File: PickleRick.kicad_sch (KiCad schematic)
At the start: 83 parts, among them J1 Conn_01x06_Male, J10 Conn_01x03_Male, J11 Conn_01x02_Male, J2 Conn_01x02_Male, J3 Conn_01x02_Male, J4 Micro_SD_Card_Det, J5 292227-7, Q1 MMDT2222A, Q2 PMV20ENR, U1 SN65HVD230, U2 ESP32-WROOM-32D, U3 MS5607-02BA

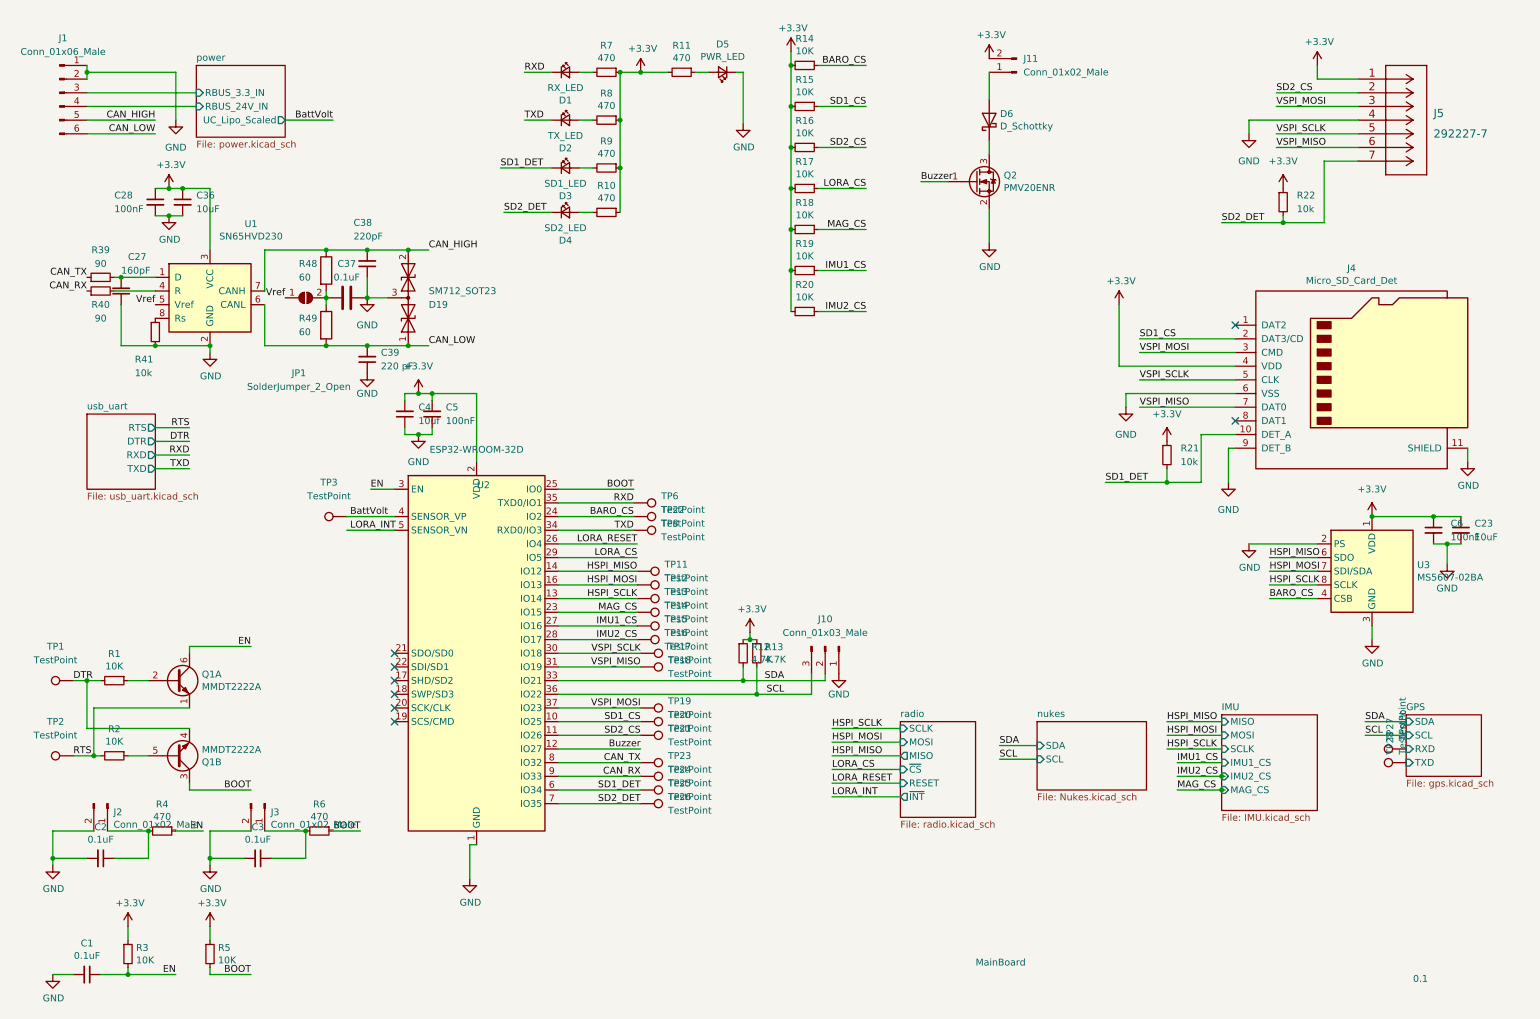
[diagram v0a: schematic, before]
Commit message: working on v2
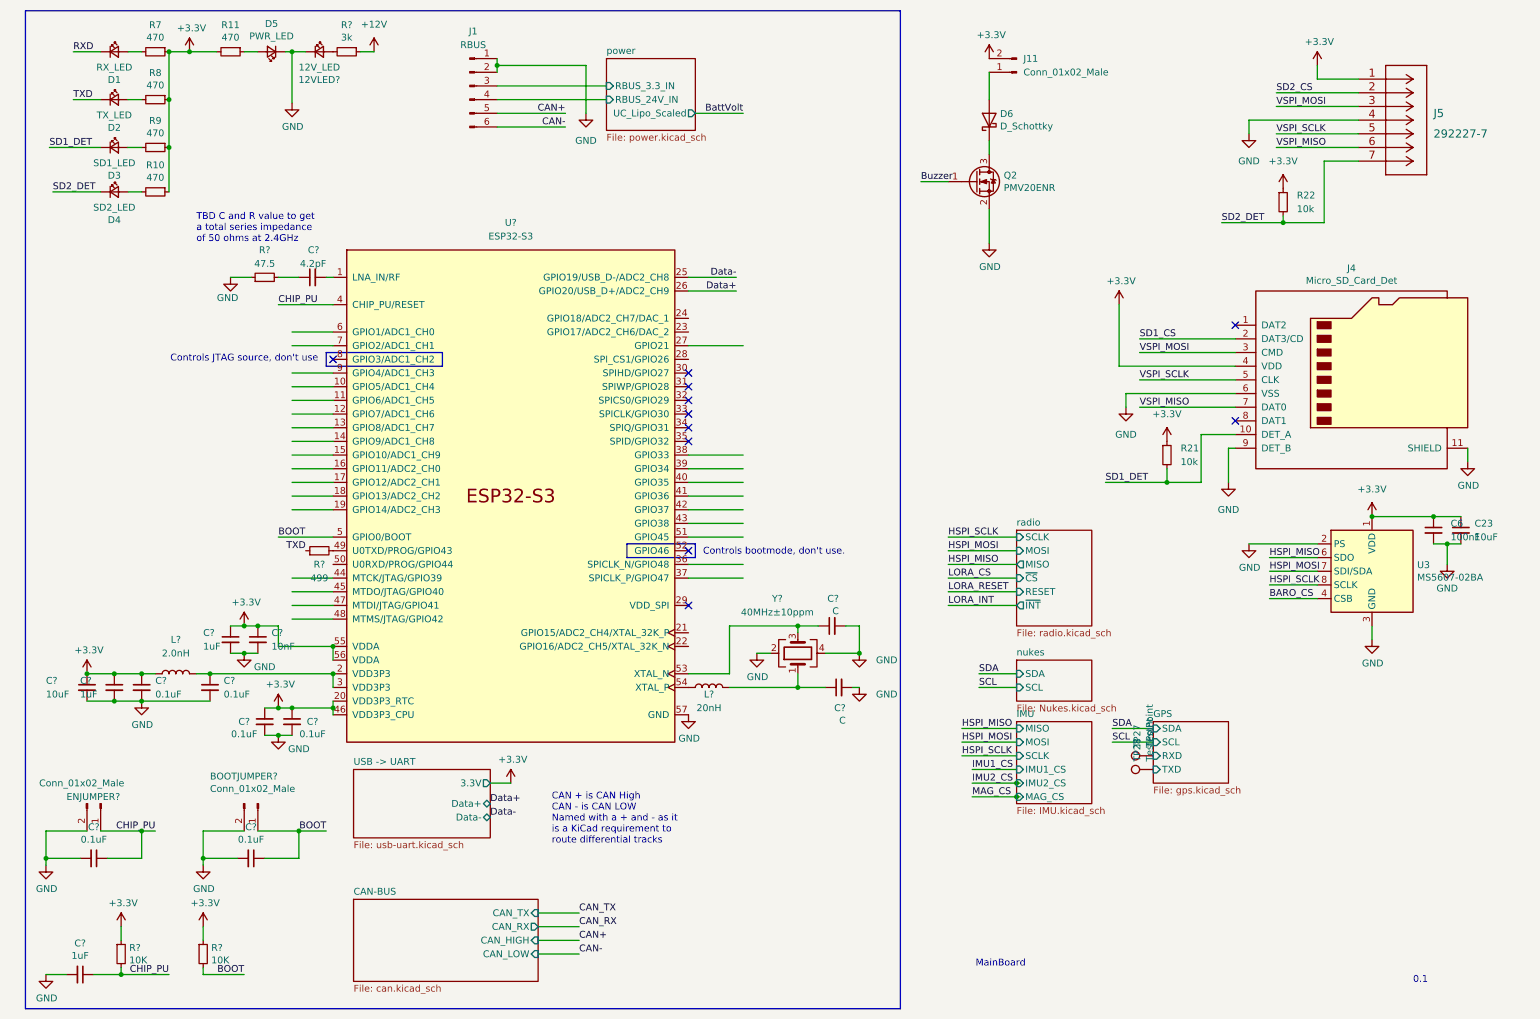
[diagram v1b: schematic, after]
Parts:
- removed C1, C2, C3: 0.1uF, Capacitor_SMD:C_0603_1608Metric, symbol Device:C_Small
- removed C27: 160pF, Capacitor_SMD:C_0603_1608Metric, symbol Device:C_Small
- removed C28, C5: 100nF, Capacitor_SMD:C_0603_1608Metric, symbol Device:C_Small
- removed C36: 10uF, Capacitor_SMD:C_0603_1608Metric, symbol Device:C_Small
- removed C37: 0.1uF, Capacitor_SMD:C_0603_1608Metric, symbol Device:C
- removed C38: 220pF, Capacitor_SMD:C_0603_1608Metric, symbol Device:C_Small
- removed C39: 220 pF, Capacitor_SMD:C_0603_1608Metric, symbol Device:C_Small
- removed C4: 10uf, Capacitor_SMD:C_0603_1608Metric, symbol Device:C_Small
- removed D19: SM712_SOT23, Package_TO_SOT_SMD:SOT-23, symbol Diode:SM712_SOT23
- removed J10: Conn_01x03_Male, Connector_PinHeader_2.54mm:PinHeader_1x03_P2.54mm_Vertical, symbol Connector:Conn_01x03_Male
- removed J2, J3: Conn_01x02_Male, Connector_PinHeader_2.54mm:PinHeader_1x02_P2.54mm_Vertical, symbol Connector:Conn_01x02_Male
- removed JP1: SolderJumper_2_Open, Jumper:SolderJumper-2_P1.3mm_Open_RoundedPad1.0x1.5mm, symbol Jumper:SolderJumper_2_Open
- removed Q1: MMDT2222A, Package_TO_SOT_SMD:SOT-363_SC-70-6, symbol Transistor_BJT:MMDT2222A
- removed R1, R14, R15, R16, R17, R18, R19, R2, R20, R3, R5: 10K, Resistor_SMD:R_0603_1608Metric, symbol Device:R_Small
- removed R12, R13: 4.7K, Resistor_SMD:R_0603_1608Metric, symbol Device:R_Small
- removed R39, R40: 90, Resistor_SMD:R_0603_1608Metric, symbol Device:R_Small
- removed R4, R6: 470, Resistor_SMD:R_0603_1608Metric, symbol Device:R_Small
- removed R41: 10k, Resistor_SMD:R_0603_1608Metric, symbol Device:R_Small
- removed R48, R49: 60, Resistor_SMD:R_0603_1608Metric, symbol Device:R
- removed TP1, TP11, TP12, TP13, TP14, TP15, TP16, TP17, TP18, TP19, TP2, TP20, TP21, TP22, TP23, TP24, TP25, TP26, TP3, TP6, TP8: TestPoint, TestPoint:TestPoint_Pad_D1.0mm, symbol Connector:TestPoint
- removed U1: SN65HVD230, Package_SO:SOIC-8_3.9x4.9mm_P1.27mm, symbol Interface_CAN_LIN:SN65HVD230
- removed U2: ESP32-WROOM-32D, RF_Module:ESP32-WROOM-32, symbol RF_Module:ESP32-WROOM-32
- added 12VLED?: 12V_LED, Resistor_SMD:R_0402_1005Metric, symbol Device:LED_Small
- added BOOTJUMPER?, ENJUMPER?: Conn_01x02_Male, Connector_PinHeader_2.54mm:PinHeader_1x02_P2.54mm_Vertical, symbol Connector:Conn_01x02_Male
- added C? (x3): 1uF, Capacitor_SMD:C_0402_1005Metric, symbol Device:C_Small
- added C? (x6): 0.1uF, Capacitor_SMD:C_0402_1005Metric, symbol Device:C_Small
- added C?: 4.2pF, Capacitor_SMD:C_0402_1005Metric, symbol Device:C_Small
- added C?: 10nF, Capacitor_SMD:C_0402_1005Metric, symbol Device:C_Small
- added C? (x2): C, Capacitor_SMD:C_0402_1005Metric, symbol Device:C_Small
- added C?: 10uF, Capacitor_SMD:C_0402_1005Metric, symbol Device:C_Small
- added L?: 2.0nH, Inductor_SMD:L_0402_1005Metric, symbol Device:L
- added L?: 20nH, Inductor_SMD:L_0402_1005Metric, symbol Device:L
- added R?: 47.5, Resistor_SMD:R_0402_1005Metric, symbol Device:R_Small
- added R? (x2): 10K, Resistor_SMD:R_0402_1005Metric, symbol Device:R_Small
- added R?: 499, Resistor_SMD:R_0402_1005Metric, symbol Device:R_Small
- added R?: 3k, Resistor_SMD:R_0402_1005Metric, symbol Device:R_Small
- added U?: ESP32-S3, Package_DFN_QFN:QFN-56-1EP_7x7mm_P0.4mm_EP5.6x5.6mm, symbol Espressif:ESP32-S3
- added Y?: 40MHz±10ppm, Crystal:Crystal_SMD_2016-4Pin_2.0x1.6mm, symbol Device:Crystal_GND24
- J1: value Conn_01x06_Male -> RBUS
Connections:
- net +3V3: now also C?.1, C?.1, C?.1, C?.1, C?.1, C?.1, C?.1, L?.1, R?.1, R?.1, U?.20 (VDD3P3_RTC), U?.46 (VDD3P3_CPU), U?.55 (VDDA), U?.56 (VDDA)
- net BOOT: now also BOOTJUMPER?.1 (Pin_1), C?.1, R?.2, U?.5 (GPIO0/BOOT)
- net GND: now also 12VLED?.1 (K), BOOTJUMPER?.2 (Pin_2), C?.2, C?.2, C?.2, C?.2, C?.2, C?.2, C?.2, C?.2, C?.2, C?.2, C?.2, C?.2, C?.2, ENJUMPER?.2 (Pin_2), R?.1, U?.57 (GND), Y?.2, Y?.4
- net TXD: now also R?.1
- net CAN_HIGH renamed CAN+
- net CAN_LOW renamed CAN-
- new net: C?.1, L?.2, U?.2 (VDD3P3), U?.3 (VDD3P3)
- new net: C?.1, R?.2
- new net: C?.2, U?.1 (LNA_IN/RF)
- new net: R?.2, U?.49 (U0TXD/PROG/GPIO43)
- new net: C?.1, U?.53 (XTAL_N), Y?.3
- new net: L?.1, U?.54 (XTAL_P)
- new net: C?.1, L?.2, Y?.1
- new net: 12VLED?.2 (A), R?.2
- new net +12V: R?.1
- new net CHIP_PU: C?.1, C?.1, ENJUMPER?.1 (Pin_1), R?.2, U?.4 (CHIP_PU/RESET)
- new net Data+: U?.26 (GPIO20/USB_D+/ADC2_CH9)
- new net Data-: U?.25 (GPIO19/USB_D-/ADC2_CH8)
- no-connect marks 8 -> 11
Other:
- removed sheet usb_uart
- added sheet CAN-BUS (can.kicad_sch)
- added sheet USB -> UART (usb-uart.kicad_sch)
- note added: "CAN + is CAN High CAN - is CAN LOW Named with a + and - as it is a KiCad requirement to route differential tracks"
- note added: "Controls JTAG source, don't use"
- note added: "Controls bootmode, don't use."
- note added: "TBD C and R value to get a total series impedance of 50 ohms at 2.4GHz"
- moved on the sheet: D1, D2, D3, D4, D5, J1, R10, R11, R7, R8, R9, TP27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

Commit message: v2 time
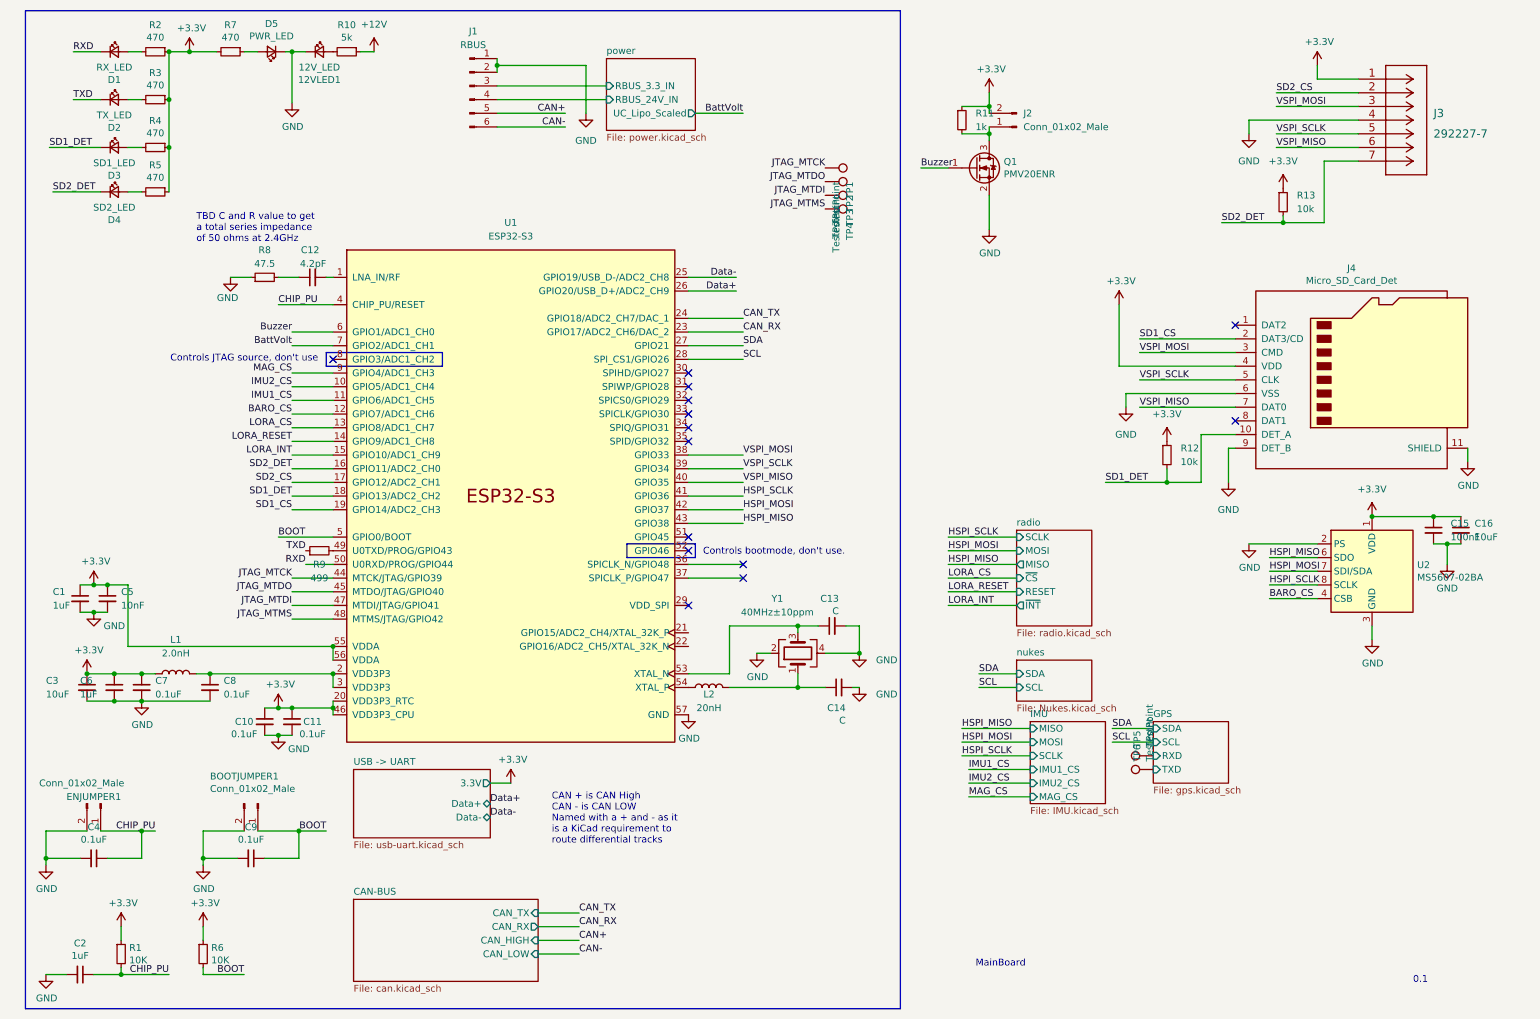
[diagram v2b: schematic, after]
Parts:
- removed D6: D_Schottky, Diode_SMD:D_SOD-123F, symbol Device:D_Schottky
- added R11: 1k, Resistor_SMD:R_0402_1005Metric, symbol Device:R_Small
- added TP1, TP2, TP3, TP4: TestPoint, TestPoint:TestPoint_Pad_D1.0mm, symbol Connector:TestPoint
- C15: renamed from C6; footprint Capacitor_SMD:C_0603_1608Metric -> Capacitor_SMD:C_0402_1005Metric
- C16: renamed from C23; footprint Capacitor_SMD:C_0603_1608Metric -> Capacitor_SMD:C_0402_1005Metric
- D1, D2, D3, D4, D5: footprint LED_SMD:LED_0603_1608Metric -> LED_SMD:LED_0402_1005Metric
- R10: renamed from R?; value 3k -> 5k; footprint Resistor_SMD:R_0402_1005Metric -> Resistor_SMD:R_0603_1608Metric
- R12: renamed from R21; footprint Resistor_SMD:R_0603_1608Metric -> Resistor_SMD:R_0402_1005Metric
- R13: renamed from R22; footprint Resistor_SMD:R_0603_1608Metric -> Resistor_SMD:R_0402_1005Metric
- R2: renamed from R7; footprint Resistor_SMD:R_0603_1608Metric -> Resistor_SMD:R_0402_1005Metric
- R3: renamed from R8; footprint Resistor_SMD:R_0603_1608Metric -> Resistor_SMD:R_0402_1005Metric
- R4: renamed from R9; footprint Resistor_SMD:R_0603_1608Metric -> Resistor_SMD:R_0402_1005Metric
- R5: renamed from R10; footprint Resistor_SMD:R_0603_1608Metric -> Resistor_SMD:R_0402_1005Metric
- R7: renamed from R11; footprint Resistor_SMD:R_0603_1608Metric -> Resistor_SMD:R_0402_1005Metric
- gave numbers to parts that had none: 25
- renumbered J11 to J2, J5 to J3, Q2 to Q1, TP27 to TP5, TP28 to TP6, U3 to U2
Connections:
- net +3V3: now also R11.1
- net BARO_CS: now also U1.12 (GPIO7/ADC1_CH6)
- net BattVolt: now also U1.7 (GPIO2/ADC1_CH1)
- net Buzzer: now also U1.6 (GPIO1/ADC1_CH0)
- net CAN_RX: now also U1.23 (GPIO17/ADC2_CH6/DAC_2)
- net CAN_TX: now also U1.24 (GPIO18/ADC2_CH7/DAC_1)
- net HSPI_MISO: now also U1.43 (GPIO38)
- net HSPI_MOSI: now also U1.42 (GPIO37)
- net HSPI_SCLK: now also U1.41 (GPIO36)
- net IMU1_CS: now also U1.11 (GPIO6/ADC1_CH5)
- net IMU2_CS: now also U1.10 (GPIO5/ADC1_CH4)
- net LORA_CS: now also U1.13 (GPIO8/ADC1_CH7)
- net LORA_INT: now also U1.15 (GPIO10/ADC1_CH9)
- net LORA_RESET: now also U1.14 (GPIO9/ADC1_CH8)
- net MAG_CS: now also U1.9 (GPIO4/ADC1_CH3)
- net RXD: now also U1.50 (U0RXD/PROG/GPIO44)
- net SCL: now also U1.28 (SPI_CS1/GPIO26)
- net SD1_CS: now also U1.19 (GPIO14/ADC2_CH3)
- net SD1_DET: now also U1.18 (GPIO13/ADC2_CH2)
- net SD2_CS: now also U1.17 (GPIO12/ADC2_CH1)
- net SD2_DET: now also U1.16 (GPIO11/ADC2_CH0)
- net SDA: now also U1.27 (GPIO21)
- net VSPI_MISO: now also U1.40 (GPIO35)
- net VSPI_MOSI: now also U1.38 (GPIO33)
- net VSPI_SCLK: now also U1.39 (GPIO34)
- net at J2.1 (Pin_1): now also Q1.3 (D), R11.2
- net JTAG_MTCK: now reaches U1.44 (MTCK/JTAG/GPIO39)
- net JTAG_MTCK: now also TP1.1
- net JTAG_MTDO: now reaches U1.45 (MTDO/JTAG/GPIO40)
- net JTAG_MTDO: now also TP2.1
- net JTAG_MTDI: now reaches U1.47 (MTDI/JTAG/GPIO41)
- net JTAG_MTDI: now also TP3.1
- net JTAG_MTMS: now reaches U1.48 (MTMS/JTAG/GPIO42)
- net JTAG_MTMS: now also TP4.1
- no-connect marks 11 -> 14
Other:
- moved on the sheet: C1, C5, J2, Q1
